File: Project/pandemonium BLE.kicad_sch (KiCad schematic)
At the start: 123 parts, among them J5 SWD_TC2030, SW1 RotaryEncoder_Switch, SW2 RotaryEncoder_Switch, SW44 RST, U1 nRF52840, Y1 32.768 KHz, Y2 32 MHz

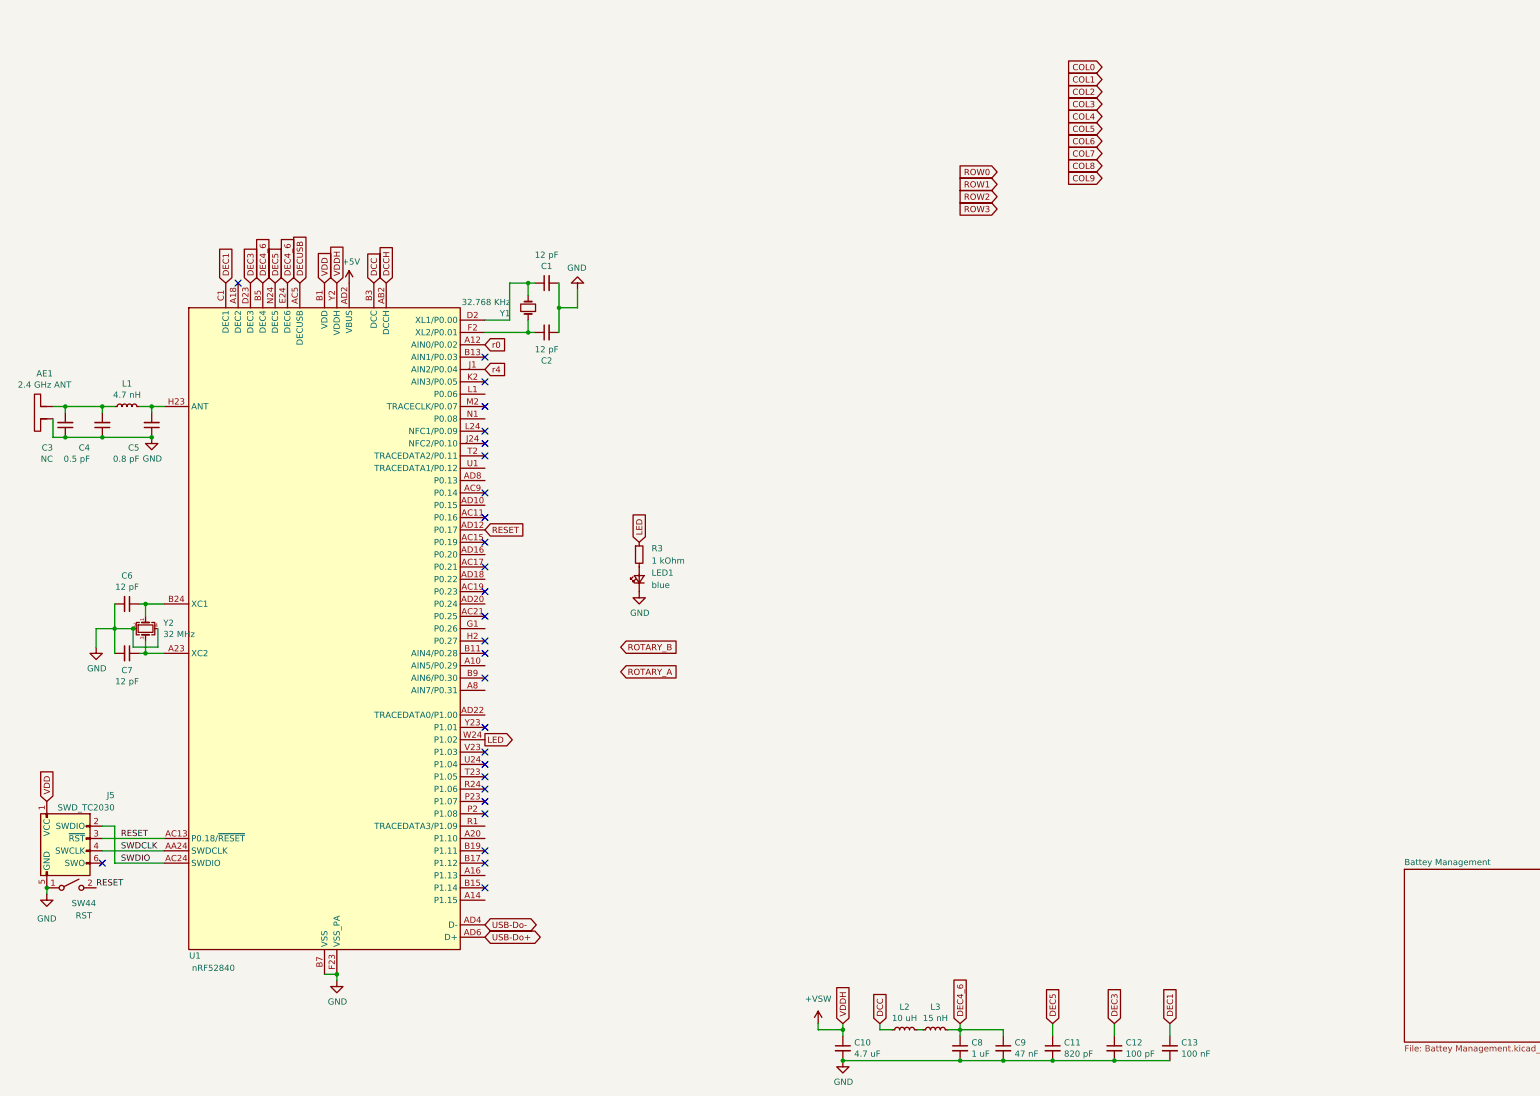
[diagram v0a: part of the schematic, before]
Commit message: EC version finished
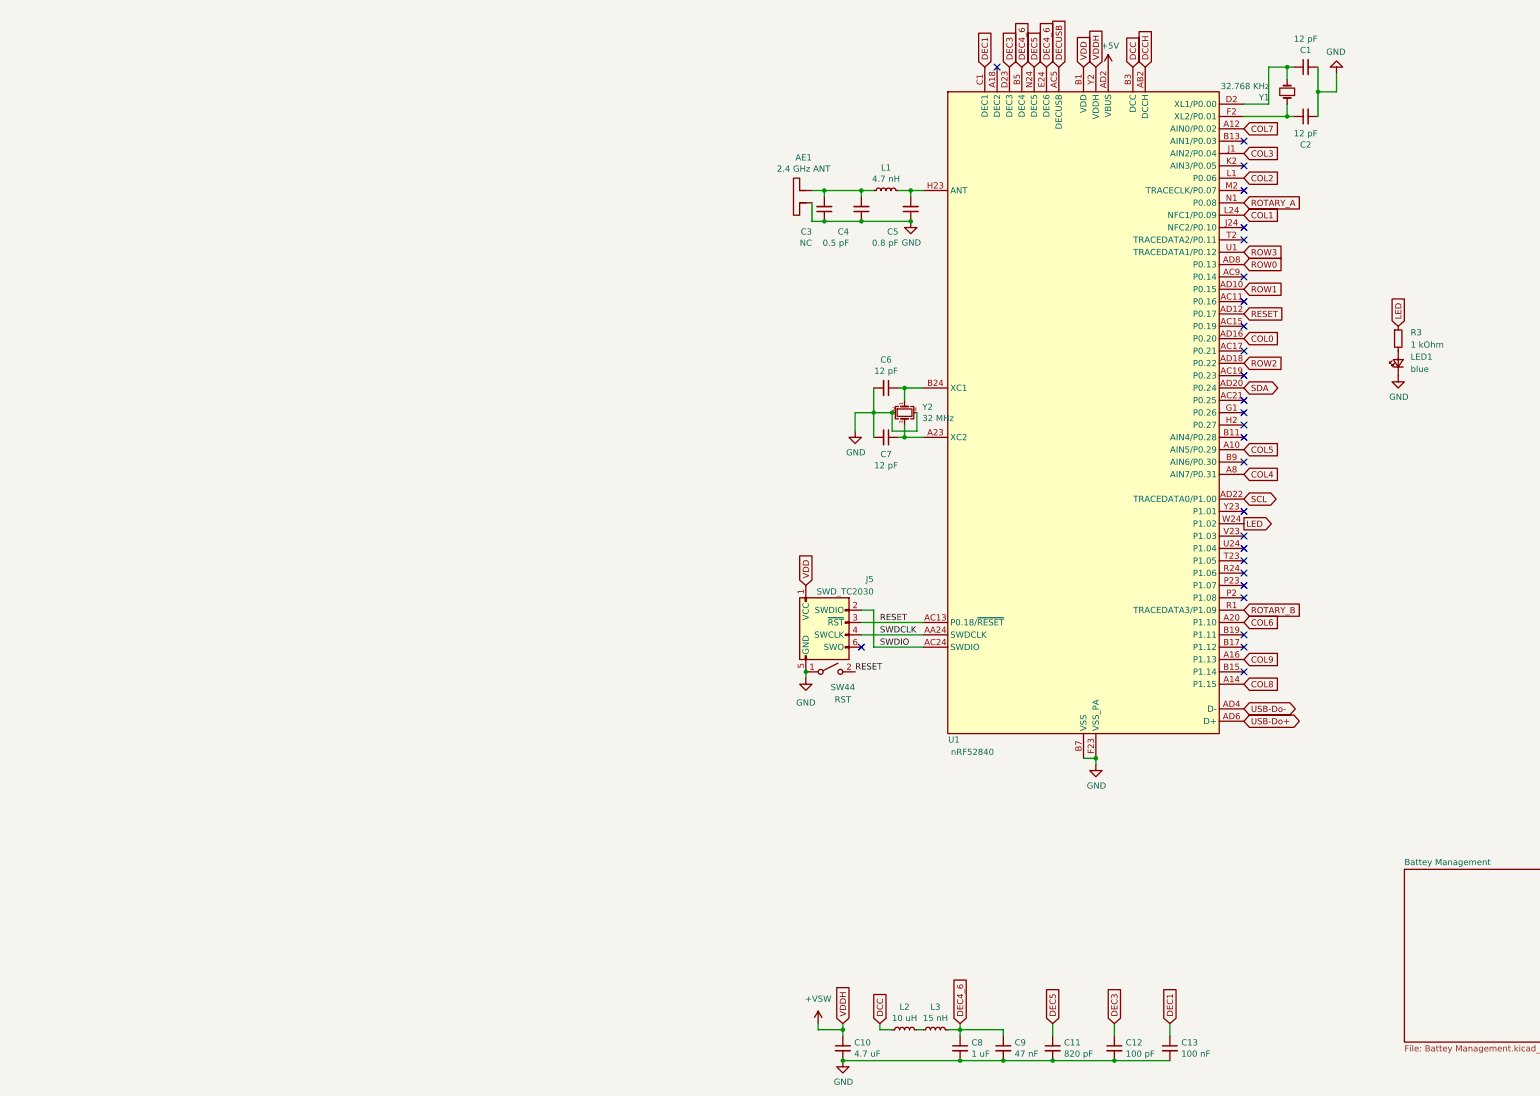
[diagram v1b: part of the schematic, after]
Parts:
- SW44: footprint PCM_marbastlib-various:SW_SPST_SKQG_WithStem -> Button_Switch_SMD:SW_Push_SPST_NO_Alps_SKRK
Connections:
- net r0 is gone; now on net COL7: U1.A12 (AIN0/P0.02)
- net r4 is gone; now on net COL3: U1.J1 (AIN2/P0.04)
- net COL0: now also U1.AD16 (P0.20)
- net COL1: now also U1.L24 (NFC1/P0.09)
- net COL2: now also U1.L1 (P0.06)
- net COL4: now also U1.A8 (AIN7/P0.31)
- net COL5: now also U1.A10 (AIN5/P0.29)
- net COL6: now also U1.A20 (P1.10)
- net COL8: now also U1.A14 (P1.15)
- net COL9: now also U1.A16 (P1.13)
- net ROTARY_A: now also U1.N1 (P0.08)
- net ROTARY_B: now also U1.R1 (TRACEDATA3/P1.09)
- net ROW0: now also U1.AD8 (P0.13)
- net ROW1: now also U1.AD10 (P0.15)
- net ROW2: now also U1.AD18 (P0.22)
- net ROW3: now also U1.U1 (TRACEDATA1/P0.12)
- net SDA: now reaches U1.AD20 (P0.24)
- net SCL: now reaches U1.AD22 (TRACEDATA0/P1.00)
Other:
- moved on the sheet: AE1, C1, C2, C3, C4, C5, C6, C7, J5, L1, LED1, R3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
